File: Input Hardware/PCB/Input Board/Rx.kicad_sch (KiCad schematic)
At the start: 32 parts

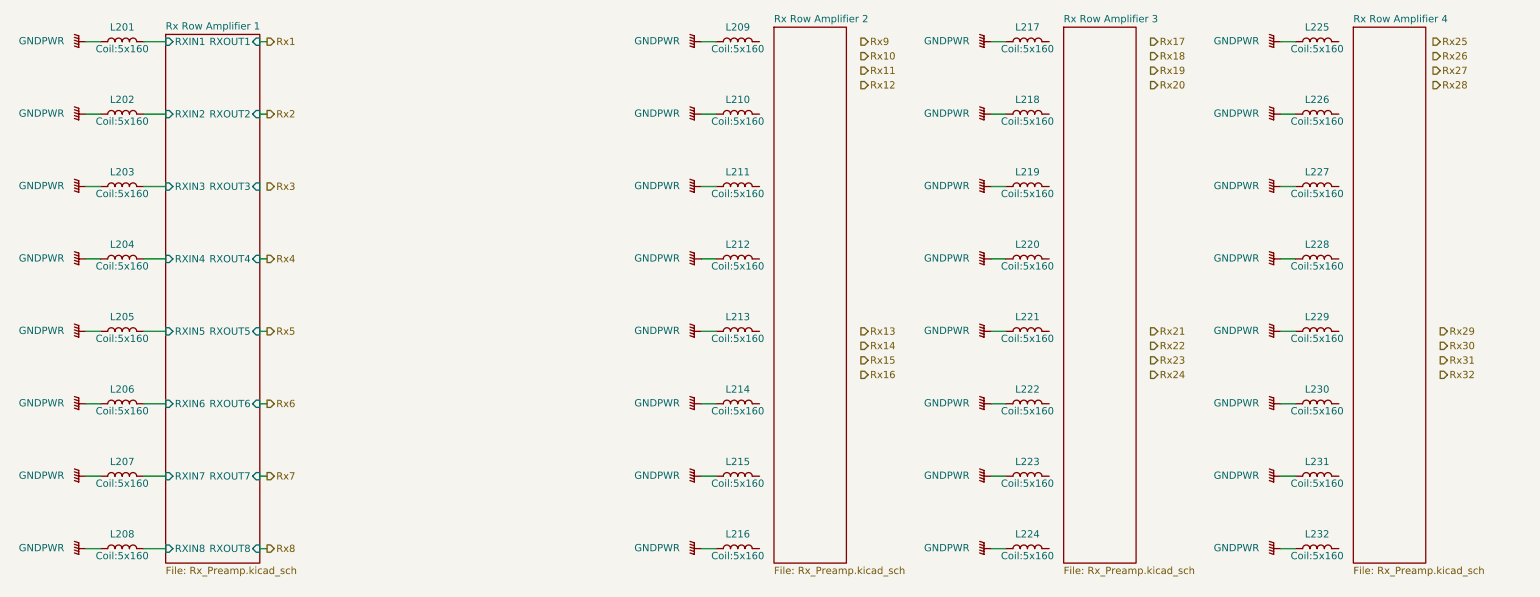
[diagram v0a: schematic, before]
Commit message: explosion 💥
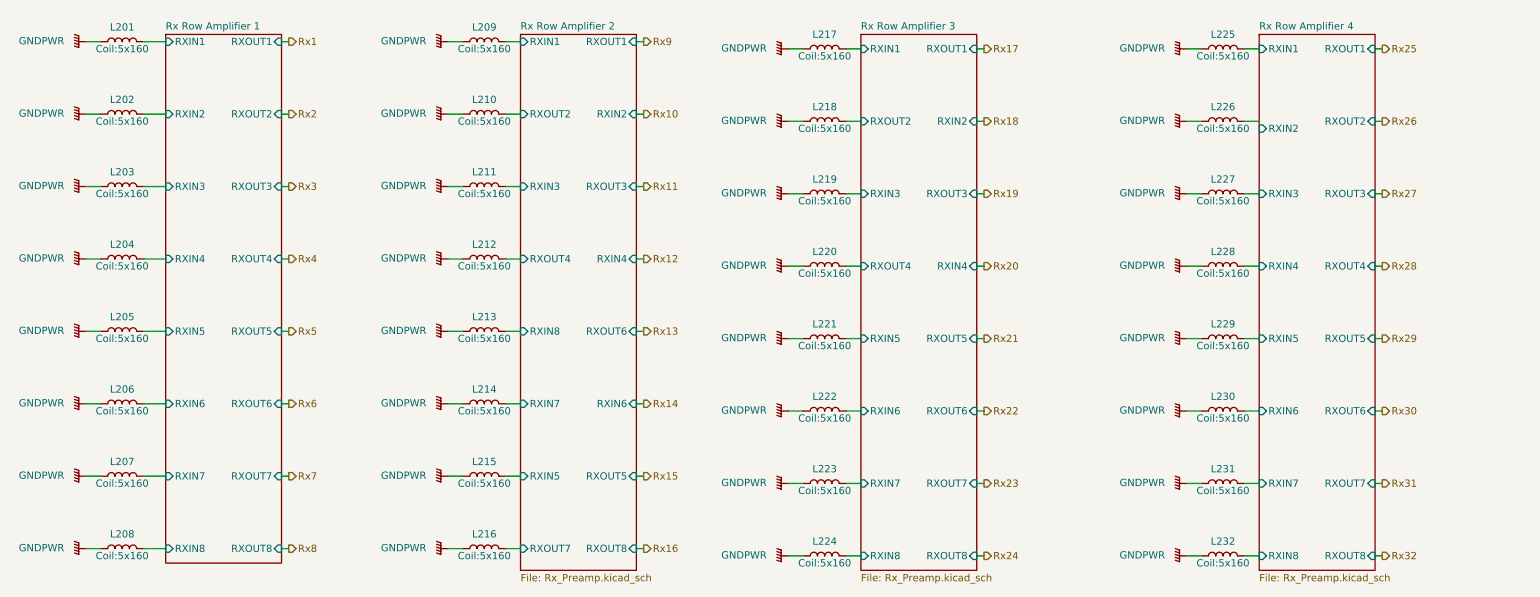
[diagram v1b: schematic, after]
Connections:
- net Rx Row Amplifier 4/RXIN4: now reaches L228.2
- net Rx Row Amplifier 2/RXOUT4: now reaches L212.2
- net Rx Row Amplifier 4/RXIN6: now reaches L230.2
- net Rx Row Amplifier 2/RXIN8: now reaches L213.2
- net Rx Row Amplifier 3/RXIN3: now reaches L219.2
- net Rx Row Amplifier 3/RXIN1: now reaches L217.2
- net Rx Row Amplifier 4/RXIN7: now reaches L231.2
- net Rx Row Amplifier 2/RXOUT2: now reaches L210.2
- net Rx Row Amplifier 2/RXIN1: now reaches L209.2
- net Rx Row Amplifier 4/RXIN5: now reaches L229.2
- net Rx Row Amplifier 4/RXIN1: now reaches L225.2
- net Rx Row Amplifier 3/RXIN5: now reaches L221.2
- net Rx Row Amplifier 3/RXIN7: now reaches L223.2
- net Rx Row Amplifier 4/RXIN3: now reaches L227.2
- net Rx Row Amplifier 4/RXIN8: now reaches L232.2
- net Rx Row Amplifier 3/RXOUT4: now reaches L220.2
- net Rx Row Amplifier 2/RXIN7: now reaches L214.2
- net Rx Row Amplifier 2/RXOUT7: now reaches L216.2
- net Rx Row Amplifier 3/RXIN6: now reaches L222.2
- net Rx Row Amplifier 3/RXOUT2: now reaches L218.2
- net Rx Row Amplifier 3/RXIN8: now reaches L224.2
- net Rx Row Amplifier 2/RXIN5: now reaches L215.2
- net Rx Row Amplifier 2/RXIN3: now reaches L211.2
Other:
- sheet Rx Row Amplifier 2 ports: added RXIN1, RXIN2, RXIN3, RXIN4, RXIN5, RXIN6, RXIN7, RXIN8, RXOUT1, RXOUT2, RXOUT3, RXOUT4, RXOUT5, RXOUT6, RXOUT7, RXOUT8; removed none
- sheet Rx Row Amplifier 3 ports: added RXIN1, RXIN2, RXIN3, RXIN4, RXIN5, RXIN6, RXIN7, RXIN8, RXOUT1, RXOUT2, RXOUT3, RXOUT4, RXOUT5, RXOUT6, RXOUT7, RXOUT8; removed none
- sheet Rx Row Amplifier 4 ports: added RXIN1, RXIN2, RXIN3, RXIN4, RXIN5, RXIN6, RXIN7, RXIN8, RXOUT1, RXOUT2, RXOUT3, RXOUT4, RXOUT5, RXOUT6, RXOUT7, RXOUT8; removed none
- moved on the sheet: L209, L210, L211, L212, L213, L214, L215, L216, L217, L218, L219, L220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
